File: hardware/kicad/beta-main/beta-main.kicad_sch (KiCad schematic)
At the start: 7 parts

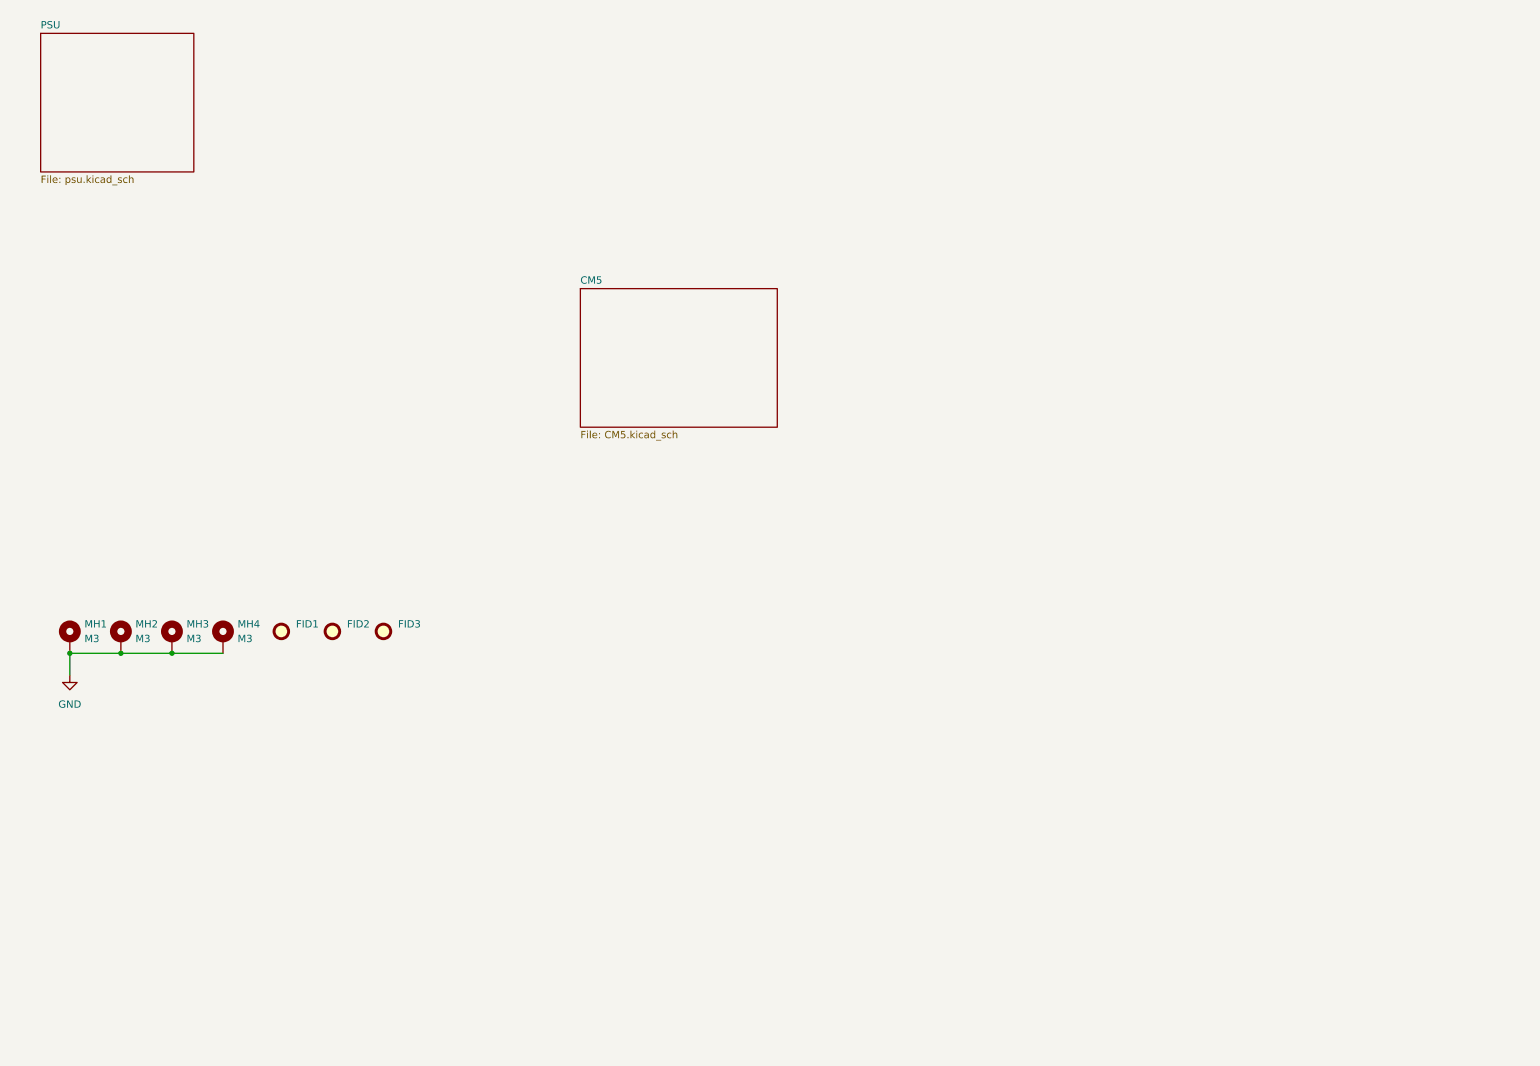
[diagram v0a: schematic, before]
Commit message: add modifications
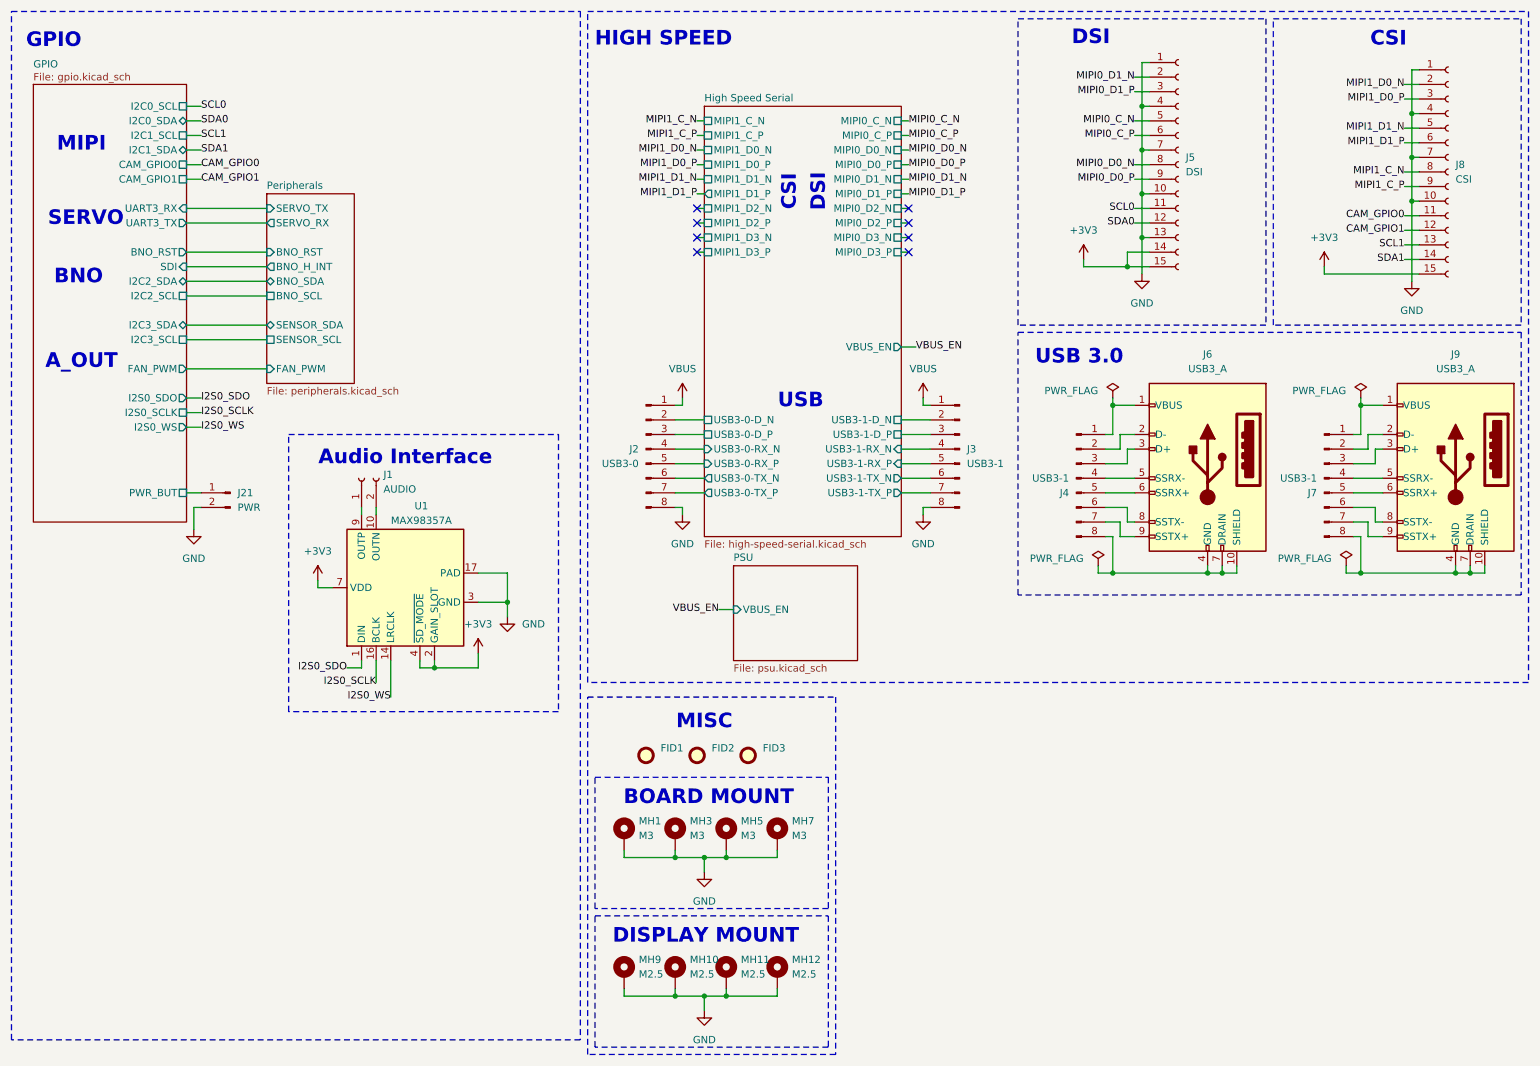
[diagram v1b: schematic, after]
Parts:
- added J1: AUDIO, Connector_JST:JST_PH_B2B-PH-K_1x02_P2.00mm_Vertical, symbol Connector:Conn_01x02_Socket
- added J2: USB3-0, Connector_JST:JST_PH_B8B-PH-K_1x08_P2.00mm_Vertical, symbol Connector:Conn_01x08_Pin
- added J21: PWR, Connector_JST:JST_PH_B2B-PH-K_1x02_P2.00mm_Vertical, symbol Connector:Conn_01x02_Pin
- added J3, J4, J7: USB3-1, Connector_JST:JST_PH_B8B-PH-K_1x08_P2.00mm_Vertical, symbol Connector:Conn_01x08_Pin
- added J5: DSI, Connector_FFC-FPC:TE_1-84953-5_1x15-1MP_P1.0mm_Horizontal, symbol Connector:Conn_01x15_Socket
- added J6, J9: USB3_A, BETA:22009L012N1, symbol Connector:USB3_A
- added J8: CSI, Connector_FFC-FPC:TE_1-84953-5_1x15-1MP_P1.0mm_Horizontal, symbol Connector:Conn_01x15_Socket
- added MH10, MH11, MH12, MH9: M2.5, MountingHole:MountingHole_2.7mm_Pad, symbol Mechanical:MountingHole_Pad
- added U1: MAX98357A, Package_DFN_QFN:TQFN-16-1EP_3x3mm_P0.5mm_EP1.23x1.23mm, symbol Beta:MAX98357A
- renumbered MH2 to MH3, MH3 to MH5, MH4 to MH7
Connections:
- net GND: now also J2.8 (Pin_8), J21.2 (Pin_2), J3.8 (Pin_8), J5.1 (Pin_1), J5.10 (Pin_10), J5.13 (Pin_13), J5.4 (Pin_4), J5.7 (Pin_7), J8.1 (Pin_1), J8.10 (Pin_10), J8.4 (Pin_4), J8.7 (Pin_7), MH10.1, MH11.1, MH12.1, MH9.1, U1.11 (GND), U1.15 (GND), U1.17 (PAD), U1.3 (GND)
- new net: J1.2 (Pin_2), U1.10 (OUTN)
- new net: J1.1 (Pin_1), U1.9 (OUTP)
- new net: J4.1 (Pin_1), J6.1 (VBUS)
- new net: J4.2 (Pin_2), J6.2 (D-)
- new net: J4.3 (Pin_3), J6.3 (D+)
- new net: J4.4 (Pin_4), J6.5 (SSRX-)
- new net: J4.5 (Pin_5), J6.6 (SSRX+)
- new net: J4.6 (Pin_6), J6.8 (SSTX-)
- new net: J4.7 (Pin_7), J6.9 (SSTX+)
- new net: J4.8 (Pin_8), J6.10 (SHIELD), J6.4 (GND), J6.7 (DRAIN)
- new net: J7.1 (Pin_1), J9.1 (VBUS)
- new net: J7.8 (Pin_8), J9.10 (SHIELD), J9.4 (GND), J9.7 (DRAIN)
- new net: J7.2 (Pin_2), J9.2 (D-)
- new net: J7.3 (Pin_3), J9.3 (D+)
- new net: J7.4 (Pin_4), J9.5 (SSRX-)
- new net: J7.5 (Pin_5), J9.6 (SSRX+)
- new net: J7.6 (Pin_6), J9.8 (SSTX-)
- new net: J7.7 (Pin_7), J9.9 (SSTX+)
- new net +3V3: J5.14 (Pin_14), J5.15 (Pin_15), J8.15 (Pin_15), U1.2 (GAIN_SLOT), U1.4 (~{SD_MODE}), U1.7 (VDD), U1.8 (VDD)
- new net CAM_GPIO0: J8.11 (Pin_11)
- new net CAM_GPIO1: J8.12 (Pin_12)
- new net GPIO/PWR_BUT: J21.1 (Pin_1)
- new net High Speed Serial/USB3-0-D_N: J2.2 (Pin_2)
- new net High Speed Serial/USB3-0-D_P: J2.3 (Pin_3)
- new net High Speed Serial/USB3-0-RX_N: J2.4 (Pin_4)
- new net High Speed Serial/USB3-0-RX_P: J2.5 (Pin_5)
- new net High Speed Serial/USB3-0-TX_N: J2.6 (Pin_6)
- new net High Speed Serial/USB3-0-TX_P: J2.7 (Pin_7)
- new net High Speed Serial/USB3-1-D_N: J3.2 (Pin_2)
- new net High Speed Serial/USB3-1-D_P: J3.3 (Pin_3)
- new net High Speed Serial/USB3-1-RX_N: J3.4 (Pin_4)
- new net High Speed Serial/USB3-1-RX_P: J3.5 (Pin_5)
- new net High Speed Serial/USB3-1-TX_N: J3.6 (Pin_6)
- new net High Speed Serial/USB3-1-TX_P: J3.7 (Pin_7)
- new net I2S0_SCLK: U1.16 (BCLK)
- new net I2S0_SDO: U1.1 (DIN)
- new net I2S0_WS: U1.14 (LRCLK)
- new net MIPI0_C_N: J5.5 (Pin_5)
- new net MIPI0_C_P: J5.6 (Pin_6)
- new net MIPI0_D0_N: J5.8 (Pin_8)
- new net MIPI0_D0_P: J5.9 (Pin_9)
- new net MIPI0_D1_N: J5.2 (Pin_2)
- new net MIPI0_D1_P: J5.3 (Pin_3)
- new net MIPI1_C_N: J8.8 (Pin_8)
- new net MIPI1_C_P: J8.9 (Pin_9)
- new net MIPI1_D0_N: J8.2 (Pin_2)
- new net MIPI1_D0_P: J8.3 (Pin_3)
- new net MIPI1_D1_N: J8.5 (Pin_5)
- new net MIPI1_D1_P: J8.6 (Pin_6)
- new net SCL0: J5.11 (Pin_11)
- new net SCL1: J8.13 (Pin_13)
- new net SDA0: J5.12 (Pin_12)
- new net SDA1: J8.14 (Pin_14)
- new net VBUS: J2.1 (Pin_1), J3.1 (Pin_1)
- no-connect marks 0 -> 8
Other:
- removed sheet CM5
- added sheet GPIO (gpio.kicad_sch)
- added sheet High Speed Serial (high-speed-serial.kicad_sch)
- added sheet Peripherals (peripherals.kicad_sch)
- sheet PSU ports: added VBUS_EN; removed none
- note added: "A_OUT"
- note added: "Audio Interface"
- note added: "BNO"
- note added: "BOARD MOUNT"
- note added: "CSI"
- note added: "DISPLAY MOUNT"
- note added: "DSI"
- note added: "GPIO"
- note added: "HIGH SPEED"
- note added: "MIPI"
- note added: "MISC"
- note added: "SERVO"
- note added: "USB"
- note added: "USB 3.0"
- title: BETA MAIN BOARD -> BETA MAIN BOARD - CM5
- moved on the sheet: FID1, FID2, FID3, MH1, MH3, MH5, MH7
